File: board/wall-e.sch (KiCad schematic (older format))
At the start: 59 parts, among them J1 Raspberry_Pi_2_3, J10 PCA9685, J11 VL53L0X, J12 VL53L0X, J13 VL53L0X, J14 MotorDrv2, J15 Motor2, J16 IMU, J17 INA219, J18 INA219, J2 LogicPwr, J3 NoisyPwr, J4 SSD1351, J5 MotorDrv1, J6 Motor1, J7 VL53L0X, J8 VL53L0X, J9 VL53L0X, U1 P8X32A-Q44, U2 TCA9548A_TSSOP, U3 ISO7742, U4 ISO7742, U5 ISO1541, Y1 Crystal

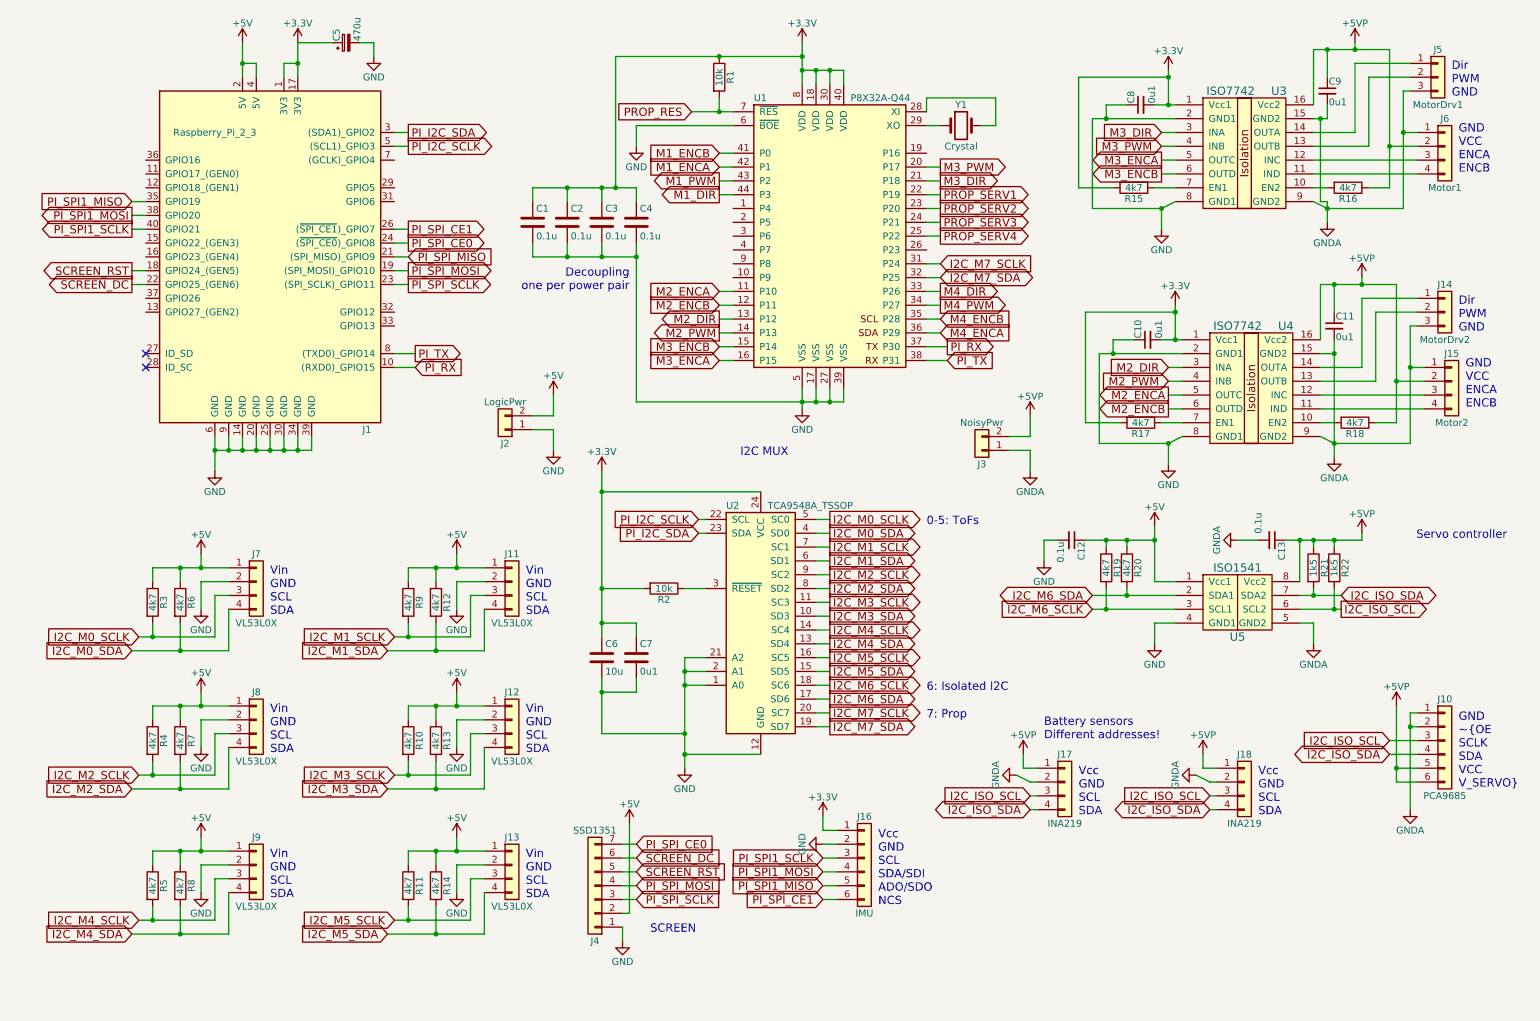
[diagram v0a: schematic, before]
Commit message: Tweaks
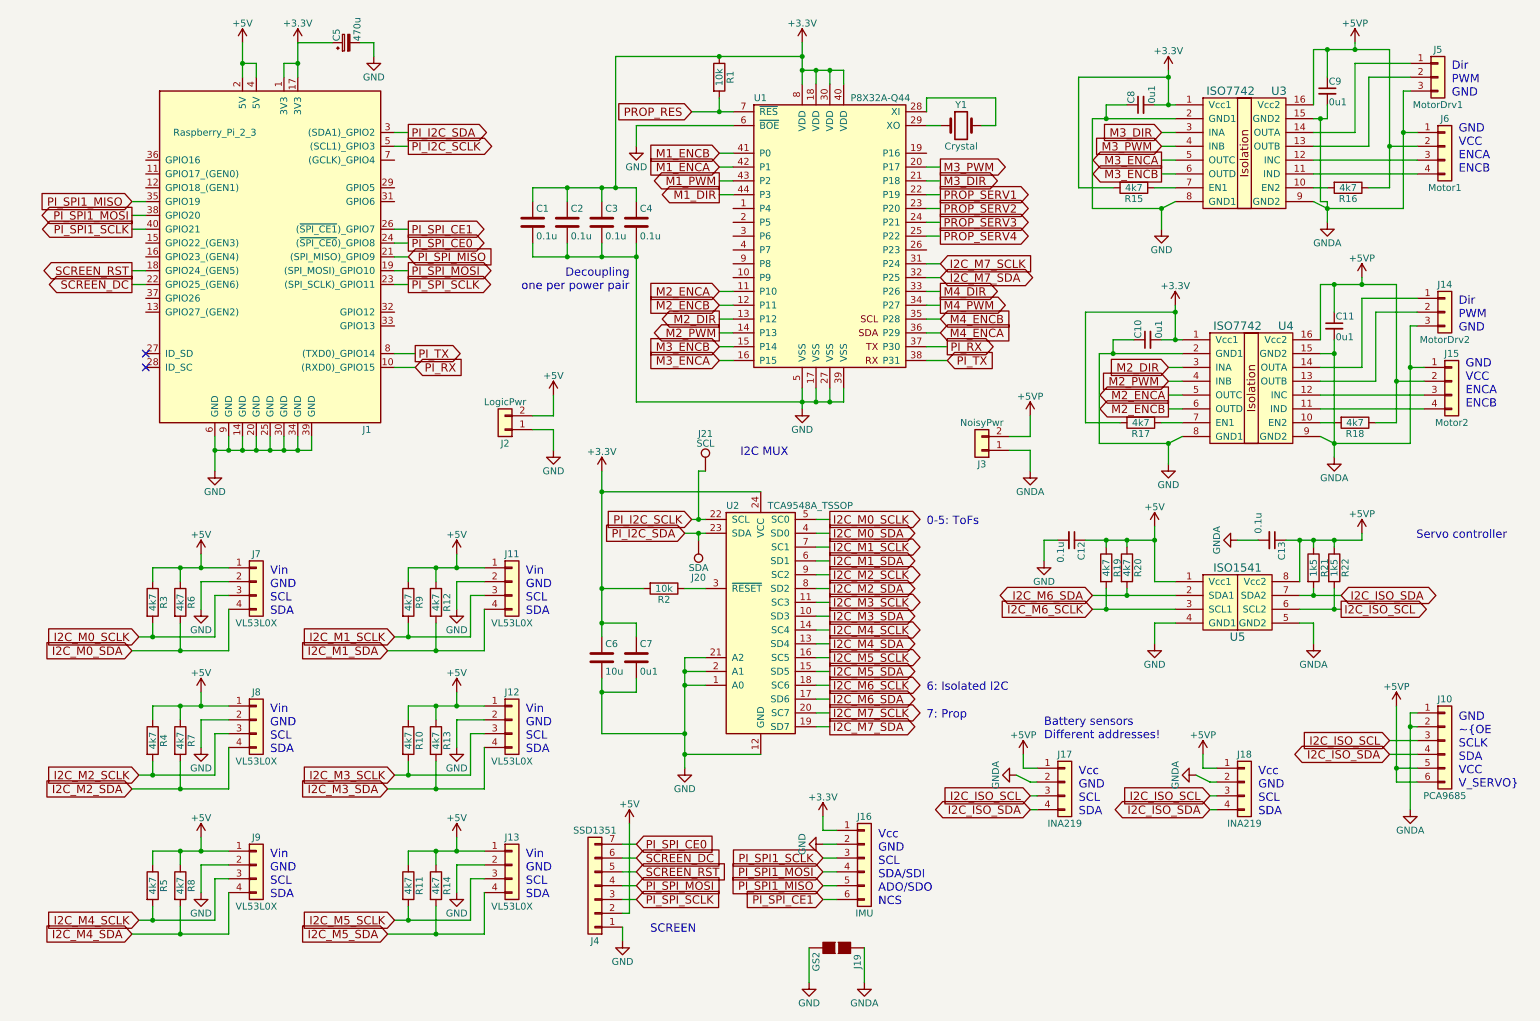
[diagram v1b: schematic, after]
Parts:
- added J19: GS2, Connectors:GS2, symbol GS2
- added J20: SDA, symbol TEST_1P
- added J21: SCL, symbol TEST_1P
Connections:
- net GND: now also J19.2 (G2)
- net GNDA: now also J19.1 (G1)
- net PI_I2C_SCLK: now also J21.1
- net PI_I2C_SDA: now also J20.1
